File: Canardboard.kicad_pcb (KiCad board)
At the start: 4 copper layers, 56.1 x 68.5 mm, 143 parts, among them IC1 SIC437DED-T1-GE3, J1 RBUS, J2 USB_C_Receptacle_USB2.0, J3 Micro_SD_Card_Det, J4 Conn_01x02_Male, J5 Conn_01x03_Male, J6 Conn_01x03_Male, J7 Conn_01x03_Male, Q1 PXP012-30QLJ, Q10 PXP012-30QLJ, Q2 PXP012-30QLJ, Q3 PXP012-30QLJ, Q4 PXP012-30QLJ, Q5 PXP012-30QLJ, Q6 PXP012-30QLJ, Q7 PXP012-30QLJ, Q8 PXP012-30QLJ, Q9 PXP012-30QLJ, U1 ESP32-S3, U10 MP28167GQ-A-Z, U11 LTC4412xS6, U12 LTC4412xS6, U2 SN65HVD230, U3 LTC4412xS6, U4 LTC4412xS6, U5 LTC4412xS6, U7 ICM-20608-G, U8 MMC5983MA, Y1 40MHz±10ppm

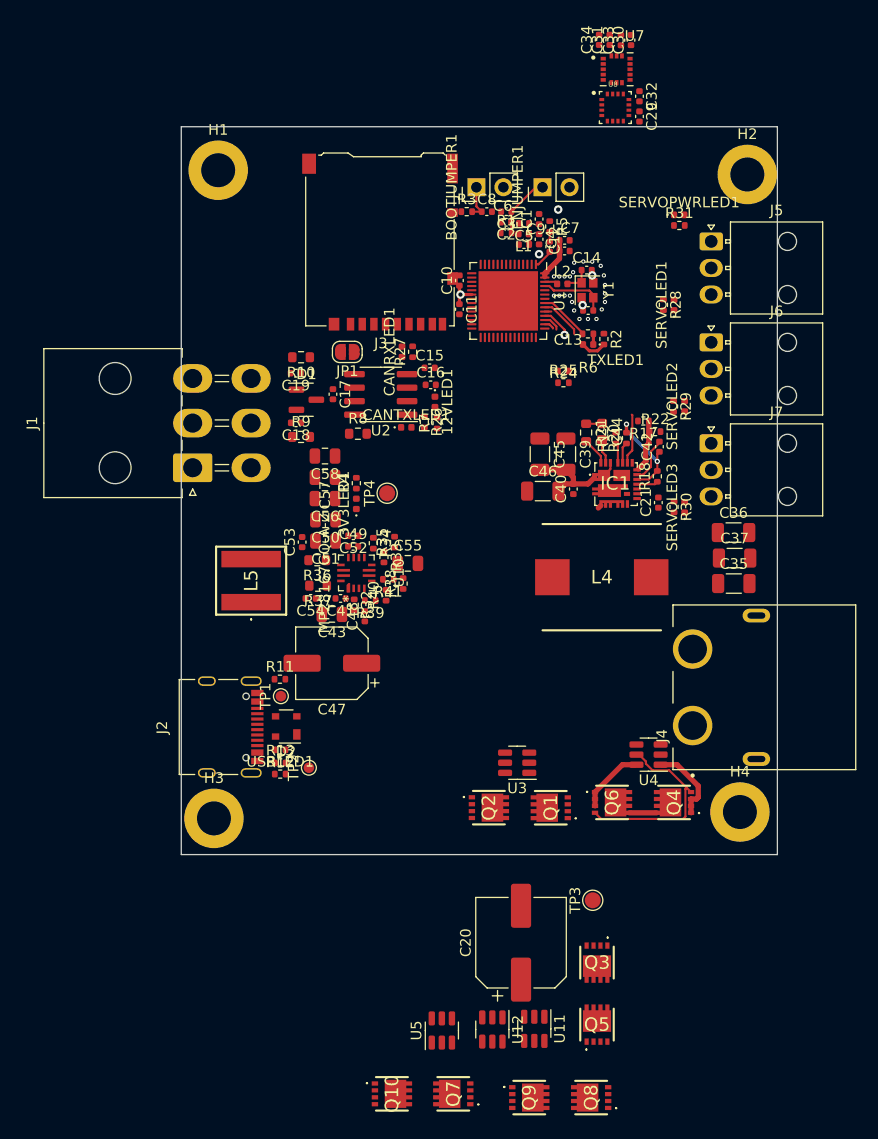
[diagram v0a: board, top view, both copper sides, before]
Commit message: I don't want to lose all my changes so I will commit, commit.
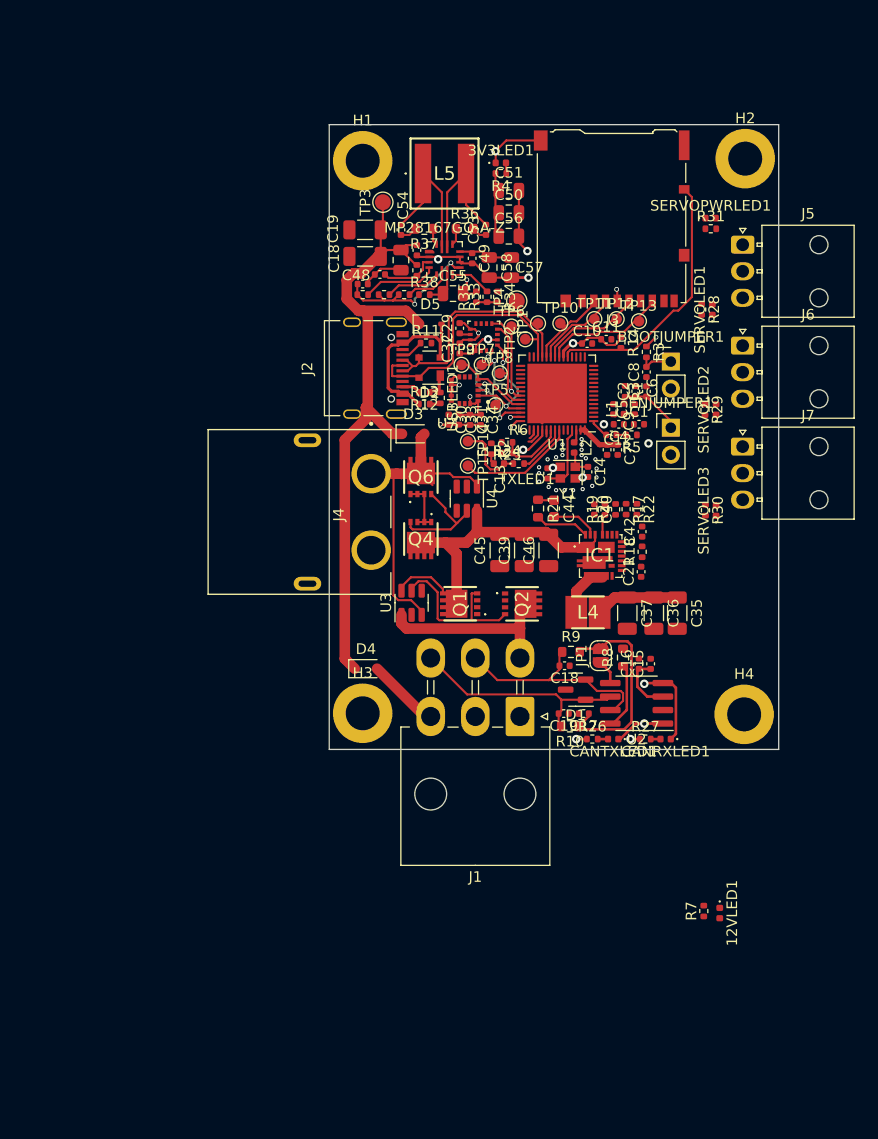
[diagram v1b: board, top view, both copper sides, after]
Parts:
- removed C20: 390uF, Capacitor_SMD:CP_Elec_8x11.9
- removed C47: 100uF, Capacitor_SMD:CP_Elec_6.3x5.4
- removed Q10, Q3, Q5, Q7, Q8, Q9: PXP012-30QLJ, iclr:PXP01230QLJ
- removed U11, U12, U5: LTC4412xS6, Package_TO_SOT_SMD:TSOT-23-6
- added C18: 47uF, Capacitor_SMD:C_1206_3216Metric, F.Cu at (104.4, 84.1)
- added C19: 47uF, Capacitor_SMD:C_1206_3216Metric, F.Cu at (104.4, 81.6)
- added D3: D_Schottky, Diode_SMD:D_SOD-323, F.Cu at (109.0, 100.8)
- added D4: D_Schottky, Diode_SMD:D_SOD-323, F.Cu at (104.5, 122.9)
- added D5: D_Schottky, Diode_SMD:D_SOD-323, F.Cu at (110.6, 90.5)
- added R14: 10k, Resistor_SMD:R_0402_1005Metric, F.Cu at (128.5, 92.2)
- added TP10: TestPoint, TestPoint:TestPoint_Pad_D1.0mm, F.Cu at (122.8, 90.4)
- added TP11: TestPoint, TestPoint:TestPoint_Pad_D1.0mm, F.Cu at (126.0, 90.0)
- added TP12: TestPoint, TestPoint:TestPoint_Pad_D1.0mm, F.Cu at (128.1, 90.0)
- added TP13: TestPoint, TestPoint:TestPoint_Pad_D1.0mm, F.Cu at (130.2, 90.2)
- added TP14: TestPoint, TestPoint:TestPoint_Pad_D1.0mm, F.Cu at (114.1, 101.5)
- added TP15: TestPoint, TestPoint:TestPoint_Pad_D1.0mm, F.Cu at (114.1, 103.8)
- added TP5: TestPoint, TestPoint:TestPoint_Pad_D1.0mm, F.Cu at (116.7, 98.1)
- added TP6: TestPoint, TestPoint:TestPoint_Pad_D1.0mm, F.Cu at (118.2, 90.7)
- added TP7: TestPoint, TestPoint:TestPoint_Pad_D1.0mm, F.Cu at (115.4, 94.3)
- added TP8: TestPoint, TestPoint:TestPoint_Pad_D1.0mm, F.Cu at (117.1, 95.1)
- added TP9: TestPoint, TestPoint:TestPoint_Pad_D1.0mm, F.Cu at (113.5, 94.3)
- L4: footprint iclr:INDPM112100X400N -> iclr:INDPM3030X200N
- moved TP3 68.6 mm to (106.1, 79.0)
- moved 12VLED1 55.1 mm to (137.8, 145.9)
- moved R7 52.3 mm to (136.3, 145.7)
- moved TP2 45.2 mm to (119.5, 91.9)
- moved CANRXLED1 44.1 mm to (132.7, 129.5), turned to 180 degrees
- moved R10 43.0 mm to (123.7, 128.3)
- moved TP1 42.6 mm to (120.7, 90.4)
- moved R27 42.5 mm to (130.8, 129.5), turned to 0 degrees
- moved L5 42.4 mm to (111.9, 76.3), turned to 0 degrees
- moved C19 40.8 mm to (123.1, 127.1)
- moved C30 39.6 mm to (112.3, 99.5), turned to -90 degrees
- moved C33 38.8 mm to (113.2, 99.5), turned to -90 degrees
- moved J1 38.7 mm to (119.0, 127.4), turned to 180 degrees
- moved USBLED1 38.5 mm to (111.5, 97.4), turned to -90 degrees
- moved C17 38.2 mm to (125.0, 127.1), turned to 180 degrees
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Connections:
- BOOTJUMPER1 pad 1: unconnected-(BOOTJUMPER1-Pin_1-Pad1) -> GND
- C31 pad 1: Net-(U7-VDD) -> +3V3
- C33 pad 1: Net-(U7-VDD) -> +3V3
- C34 pad 1: Net-(U7-VDD) -> +3V3
- IC1 pad 29: unconnected-(IC1-PGND__5-Pad29) -> GND
- J1 pad 3: VBUS -> /rbusmosfets/RBUS_3.3
- J3 pad 10: +3V3 -> /SD_DET
- J3 pad 3: /SPI_MOSI -> /SD_MOSI
- J3 pad 5: /SPI_CLK -> /SD_CLK
- J3 pad 7: /SPI_MISO -> /SD_MISO
- Q1 pad 5: Net-(Q1-D_1) -> +12V
- Q1 pad 6: Net-(Q1-D_1) -> +12V
- Q1 pad 7: Net-(Q1-D_1) -> +12V
- Q1 pad 8: Net-(Q1-D_1) -> +12V
- Q1 pad 9: Net-(Q1-D_1) -> +12V
- Q2 pad 1: +12V -> Net-(Q1-S_1)
- Q2 pad 2: +12V -> Net-(Q1-S_1)
- Q2 pad 3: +12V -> Net-(Q1-S_1)
- Q2 pad 5: Net-(Q1-D_1) -> /rbusmosfets/RBUS_DEPL
- Q2 pad 6: Net-(Q1-D_1) -> /rbusmosfets/RBUS_DEPL
- Q2 pad 7: Net-(Q1-D_1) -> /rbusmosfets/RBUS_DEPL
- Q2 pad 8: Net-(Q1-D_1) -> /rbusmosfets/RBUS_DEPL
- Q2 pad 9: Net-(Q1-D_1) -> /rbusmosfets/RBUS_DEPL
- Q4 pad 1: /rbusmosfets/BatteryPower -> Net-(Q4-S_1)
- Q4 pad 2: /rbusmosfets/BatteryPower -> Net-(Q4-S_1)
- Q4 pad 3: /rbusmosfets/BatteryPower -> Net-(Q4-S_1)
- Q4 pad 5: Net-(Q4-D_1) -> +12V
- Q4 pad 6: Net-(Q4-D_1) -> +12V
- Q4 pad 7: Net-(Q4-D_1) -> +12V
- Q4 pad 8: Net-(Q4-D_1) -> +12V
- Q4 pad 9: Net-(Q4-D_1) -> +12V
- Q6 pad 1: +12V -> Net-(Q4-S_1)
- Q6 pad 2: +12V -> Net-(Q4-S_1)
- Q6 pad 3: +12V -> Net-(Q4-S_1)
- Q6 pad 5: Net-(Q4-D_1) -> /rbusmosfets/BatteryPower
- Q6 pad 6: Net-(Q4-D_1) -> /rbusmosfets/BatteryPower
- Q6 pad 7: Net-(Q4-D_1) -> /rbusmosfets/BatteryPower
- Q6 pad 8: Net-(Q4-D_1) -> /rbusmosfets/BatteryPower
- Q6 pad 9: Net-(Q4-D_1) -> /rbusmosfets/BatteryPower
- U1 pad 19: unconnected-(U1-GPIO14/ADC2_CH3-Pad19) -> /SD_DET
- U1 pad 21: unconnected-(U1-GPIO15/ADC2_CH4/XTAL_32K_P-Pad21) -> /SD_MISO
- U1 pad 22: unconnected-(U1-GPIO16/ADC2_CH5/XTAL_32K_N-Pad22) -> /SD_CLK
- U1 pad 23: unconnected-(U1-GPIO17/ADC2_CH6/DAC_2-Pad23) -> /SD_MOSI
- U1 pad 24: unconnected-(U1-GPIO18/ADC2_CH7/DAC_1-Pad24) -> /SD_CS
- U1 pad 36: /CAN_TX -> /SPI_MISO
- U1 pad 37: /CAN_RX -> /MAG_CS
- U1 pad 38: /SD_CS -> /IMU_CS
- U1 pad 41: /SPI_MISO -> /CAN_TX
- U1 pad 42: /SERVO_SGNL2 -> /CAN_RX
- U1 pad 45: /IMU_CS -> /SERVO_SGNL2
- U1 pad 47: /MAG_CS -> unconnected-(U1-MTDI/JTAG/GPIO41-Pad47)
- U1 pad 50: unconnected-(U1-U0RXD/PROG/GPIO44-Pad50) -> /RXD
- U3 pad 1: Net-(Q1-S_1) -> /rbusmosfets/RBUS_DEPL
- U7 pad 1: Net-(U7-VDD) -> +3V3
- U7 pad 16: Net-(U7-VDD) -> +3V3
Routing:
- net RBUS_uC_V: track 0.00 -> 64.8 mm
- net GND: track 0.06 -> 48.6 mm, vias 27 -> 34
- net +3V3: track 9.69 -> 44.8 mm, vias 2 -> 8
- net /SD_DET: track 0.00 -> 24.7 mm
- net /Data+: track 0.00 -> 24.5 mm
- net /rbusmosfets/BatteryPower: track 7.48 -> 31.9 mm
- net /Data-: track 0.00 -> 22.9 mm
- net /CAN-: track 0.00 -> 21.4 mm
- net /CAN+: track 0.00 -> 20.8 mm
- net Net-(JP1-B): track 0.00 -> 19.6 mm
- net /rbusmosfets/RBUS_DEPL: track 0.00 -> 17.5 mm
- net VBUS: track 0.00 -> 15.9 mm
- net /SPI_MISO: track 0.00 -> 15.8 mm, vias 0 -> 3
- net Net-(Q1-G): track 0.00 -> 15.6 mm
- net /servopower/uC_VCC: track 0.00 -> 14.8 mm, vias 0 -> 2
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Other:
- board size 56.1 x 68.5 mm -> 42.3 x 58.8 mm
